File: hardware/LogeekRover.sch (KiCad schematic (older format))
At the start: 65 parts, among them M1 Mounting_Hole, M2 Mounting_Hole, M3 Mounting_Hole, M4 Mounting_Hole, M5 Motor, M6 Motor, M7 Motor, M8 Motor, P1 CONN_01X01, P10 CONN_01X03, P11 CONN_01X03, P12 CONN_01X01, P13 CONN_01X01, P14 CONN_01X03, P15 CONN_01X03, P16 CONN_01X01, P17 CONN_01X01, P18 CONN_01X03, P19 CONN_01X03, P2 CONN_01X03, P20 CONN_01X01, P22 CONN_01X01, P23 CONN_01X03, P24 CONN_01X03, P25 CONN_01X01, P26 CONN_02X10, P27 CONN_02X08, P28 CONN_01X01, P29 CONN_01X03, P3 CONN_01X03, P30 CONN_01X02, P31 CONN_01X02, P32 CONN_01X01, P33 CONN_01X03, P34 CONN_01X02, P35 CONN_01X01, P36 CONN_01X03, P37 CONN_02X08, P38 CONN_02X06, P39 CONN_01X01, P4 CONN_01X01, P40 CONN_01X03, P41 CONN_01X01, P42 CONN_01X03, P43 CONN_01X01, P44 CONN_01X03, P46 CONN_01X03, P47 CONN_01X02, P48 CONN_01X03, P5 CONN_01X01, P50 CONN_01X03, P52 CONN_01X03, P53 BATT CASE, P54 CONN_01X02, P6 CONN_01X03, P7 CONN_01X03, P8 CONN_01X01, P9 CONN_01X01, U1 L9110S

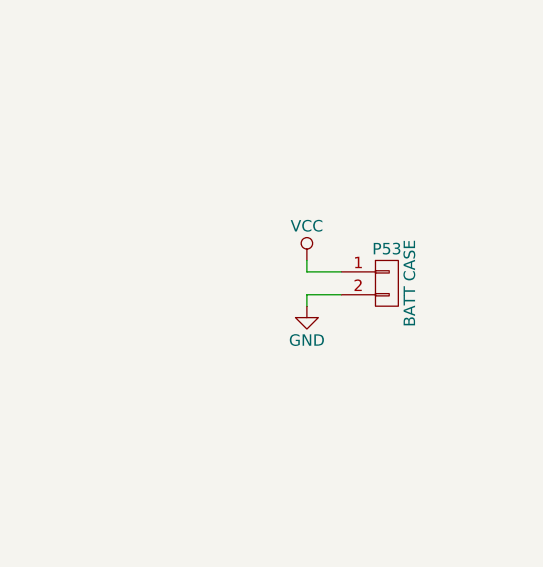
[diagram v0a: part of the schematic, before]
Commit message: Nightly Backup.
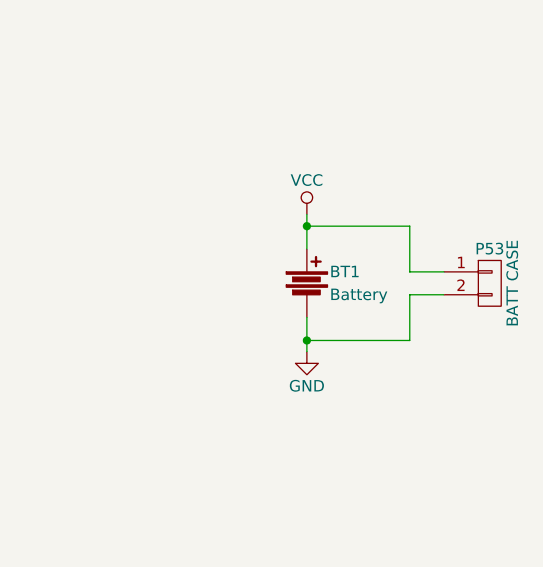
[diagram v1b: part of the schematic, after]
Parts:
- added BT1: Battery, local:Battery_Case_AAAx2, symbol Battery
- M1, M2, M3, M4: footprint Mounting_Holes:MountingHole_3mm -> local:Mounting_Hole_3mm
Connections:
- wire segments 188 -> 192
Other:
- moved on the sheet: P53
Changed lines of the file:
@@
 	2500 1000 4200 1000
 $Comp
-L VCC #PWR01
+L VCC #PWR2
 U 1 1 56A5EDCA
 P 2400 900
-F 0 "#PWR01" H 2400 750 50  0001 C CNN
+F 0 "#PWR2" H 2400 750 50  0001 C CNN
 F 1 "VCC" H 2400 1050 50  0000 C CNN
 F 2 "" H 2400 900 60  0000 C CNN
@@
 	3750 2000 3750 1900
 $Comp
-L GND #PWR02
+L GND #PWR4
 U 1 1 56A5FD75
 P 3750 2350
-F 0 "#PWR02" H 3750 2100 50  0001 C CNN
+F 0 "#PWR4" H 3750 2100 50  0001 C CNN
 F 1 "GND" H 3750 2200 50  0000 C CNN
 F 2 "" H 3750 2350 60  0000 C CNN
@@
 L CONN_01X02 P53
 U 1 1 56A607A9
-P 12550 8900
-F 0 "P53" H 12550 9050 50  0000 C CNN
-F 1 "BATT CASE" V 12650 8900 50  0000 C CNN
-F 2 "Connect:PINHEAD1-2" H 12550 8900 60  0001 C CNN
-F 3 "" H 12550 8900 60  0000 C CNN
-	1    12550 8900
-	1    0    0    -1
-$EndComp
-$Comp
-L VCC #PWR03
+P 13000 8900
+F 0 "P53" H 13000 9050 50  0000 C CNN
+F 1 "BATT CASE" V 13100 8900 50  0000 C CNN
+F 2 "Connect:PINHEAD1-2" H 13000 8900 60  0001 C CNN
+F 3 "" H 13000 8900 60  0000 C CNN
+	1    13000 8900
+	1    0    0    -1
+$EndComp
+$Comp
+L VCC #PWR8
 U 1 1 56A6091B
-P 12200 8800
-F 0 "#PWR03" H 12200 8650 50  0001 C CNN
-F 1 "VCC" H 12200 8950 50  0000 C CNN
-F 2 "" H 12200 8800 60  0000 C CNN
-F 3 "" H 12200 8800 60  0000 C CNN
-	1    12200 8800
-	1    0    0    -1
-$EndComp
-$Comp
-L GND #PWR04
+P 12200 8600
+F 0 "#PWR8" H 12200 8450 50  0001 C CNN
+F 1 "VCC" H 12200 8750 50  0000 C CNN
+F 2 "" H 12200 8600 60  0000 C CNN
+F 3 "" H 12200 8600 60  0000 C CNN
+	1    12200 8600
+	1    0    0    -1
+$EndComp
+$Comp
+L GND #PWR9
 U 1 1 56A60944
-P 12200 9000
-F 0 "#PWR04" H 12200 8750 50  0001 C CNN
-F 1 "GND" H 12200 8850 50  0000 C CNN
-F 2 "" H 12200 9000 60  0000 C CNN
-F 3 "" H 12200 9000 60  0000 C CNN
-	1    12200 9000
-	1    0    0    -1
-$EndComp
-Wire Wire Line
-	12350 8850 12200 8850
-Wire Wire Line
-	12200 8850 12200 8800
-Wire Wire Line
-	12350 8950 12200 8950
-Wire Wire Line
-	12200 8950 12200 9000
-$Comp
-L GND #PWR05
+P 12200 9200
+F 0 "#PWR9" H 12200 8950 50  0001 C CNN
+F 1 "GND" H 12200 9050 50  0000 C CNN
+F 2 "" H 12200 9200 60  0000 C CNN
+F 3 "" H 12200 9200 60  0000 C CNN
+	1    12200 9200
+	1    0    0    -1
+$EndComp
+$Comp
+L GND #PWR1
 U 1 1 56A60B6D
 P 1200 1900
-F 0 "#PWR05" H 1200 1650 50  0001 C CNN
+F 0 "#PWR1" H 1200 1650 50  0001 C CNN
 F 1 "GND" H 1200 1750 50  0000 C CNN
 F 2 "" H 1200 1900 60  0000 C CNN
@@
 5V
 $Comp
-L GND #PWR06
+L GND #PWR7
 U 1 1 56A6424E
 P 7100 8450
-F 0 "#PWR06" H 7100 8200 50  0001 C CNN
+F 0 "#PWR7" H 7100 8200 50  0001 C CNN
 F 1 "GND" H 7100 8300 50  0000 C CNN
 F 2 "" H 7100 8450 60  0000 C CNN
@@
 AREF
 $Comp
-L GND #PWR07
+L GND #PWR3
 U 1 1 56A6454B
 P 3600 7850
-F 0 "#PWR07" H 3600 7600 50  0001 C CNN
+F 0 "#PWR3" H 3600 7600 50  0001 C CNN
 F 1 "GND" H 3600 7700 50  0000 C CNN
 F 2 "" H 3600 7850 60  0000 C CNN
@@
 CLK
 $Comp
-L GND #PWR08
+L GND #PWR5
 U 1 1 56A6516D
 P 5350 7550
-F 0 "#PWR08" H 5350 7300 50  0001 C CNN
+F 0 "#PWR5" H 5350 7300 50  0001 C CNN
 F 1 "GND" H 5350 7400 50  0000 C CNN
 F 2 "" H 5350 7550 60  0000 C CNN
@@
 A5
 $Comp
-L GNDA #PWR09
+L GNDA #PWR6
 U 1 1 56A65651
 P 5500 9300
-F 0 "#PWR09" H 5500 9050 50  0001 C CNN
+F 0 "#PWR6" H 5500 9050 50  0001 C CNN
 F 1 "GNDA" H 5500 9150 50  0000 C CNN
 F 2 "" H 5500 9300 60  0000 C CNN
@@
 F 0 "M1" H 10650 1850 60  0000 C CNN
 F 1 "Mounting_Hole" H 10700 1550 60  0001 C CNN
-F 2 "Mounting_Holes:MountingHole_3mm" H 10700 1700 60  0001 C CNN
+F 2 "local:Mounting_Hole_3mm" H 10700 1700 60  0001 C CNN
 F 3 "" H 10700 1700 60  0000 C CNN
 	1    10700 1700
@@
 F 0 "M2" H 10950 1850 60  0000 C CNN
 F 1 "Mounting_Hole" H 11000 1550 60  0001 C CNN
-F 2 "Mounting_Holes:MountingHole_3mm" H 11000 1700 60  0001 C CNN
+F 2 "local:Mounting_Hole_3mm" H 11000 1700 60  0001 C CNN
 F 3 "" H 11000 1700 60  0000 C CNN
 	1    11000 1700
@@
 F 0 "M3" H 11250 1850 60  0000 C CNN
 F 1 "Mounting_Hole" H 11300 1550 60  0001 C CNN
-F 2 "Mounting_Holes:MountingHole_3mm" H 11300 1700 60  0001 C CNN
+F 2 "local:Mounting_Hole_3mm" H 11300 1700 60  0001 C CNN
 F 3 "" H 11300 1700 60  0000 C CNN
 	1    11300 1700
@@
 F 0 "M4" H 11550 1850 60  0000 C CNN
 F 1 "Mounting_Hole" H 11600 1550 60  0001 C CNN
-F 2 "Mounting_Holes:MountingHole_3mm" H 11600 1700 60  0001 C CNN
+F 2 "local:Mounting_Hole_3mm" H 11600 1700 60  0001 C CNN
 F 3 "" H 11600 1700 60  0000 C CNN
 	1    11600 1700
@@
 Wire Wire Line
 	3700 1600 4200 1600
+$Comp
+L Battery BT1
+U 1 1 56A8C54E
+P 12200 8900
+F 0 "BT1" H 12300 8950 50  0000 L CNN
+F 1 "Battery" H 12300 8850 50  0000 L CNN
+F 2 "local:Battery_Case_AAAx2" V 12200 8940 60  0001 C CNN
+F 3 "" V 12200 8940 60  0000 C CNN
+	1    12200 8900
+	1    0    0    -1
+$EndComp
+Wire Wire Line
+	12200 8600 12200 8750
+Wire Wire Line
+	12200 9050 12200 9200
+Wire Wire Line
+	12200 8650 12650 8650
+Wire Wire Line
+	12650 8650 12650 8850
+Wire Wire Line
+	12650 8850 12800 8850
+Connection ~ 12200 8650
+Wire Wire Line
+	12800 8950 12650 8950
+Wire Wire Line
+	12650 8950 12650 9150
+Wire Wire Line
+	12650 9150 12200 9150
+Connection ~ 12200 9150
 $EndSCHEMATC
